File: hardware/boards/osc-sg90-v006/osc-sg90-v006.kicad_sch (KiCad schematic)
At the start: 31 parts, among them J1 Servo Input, J2 Motor, J3 Debug, J4 Potentiometer, U1 H7133-1_C277537, U4 DRV8837, U5 CH32V006F8U6, U6 74LVC2G241GS,115

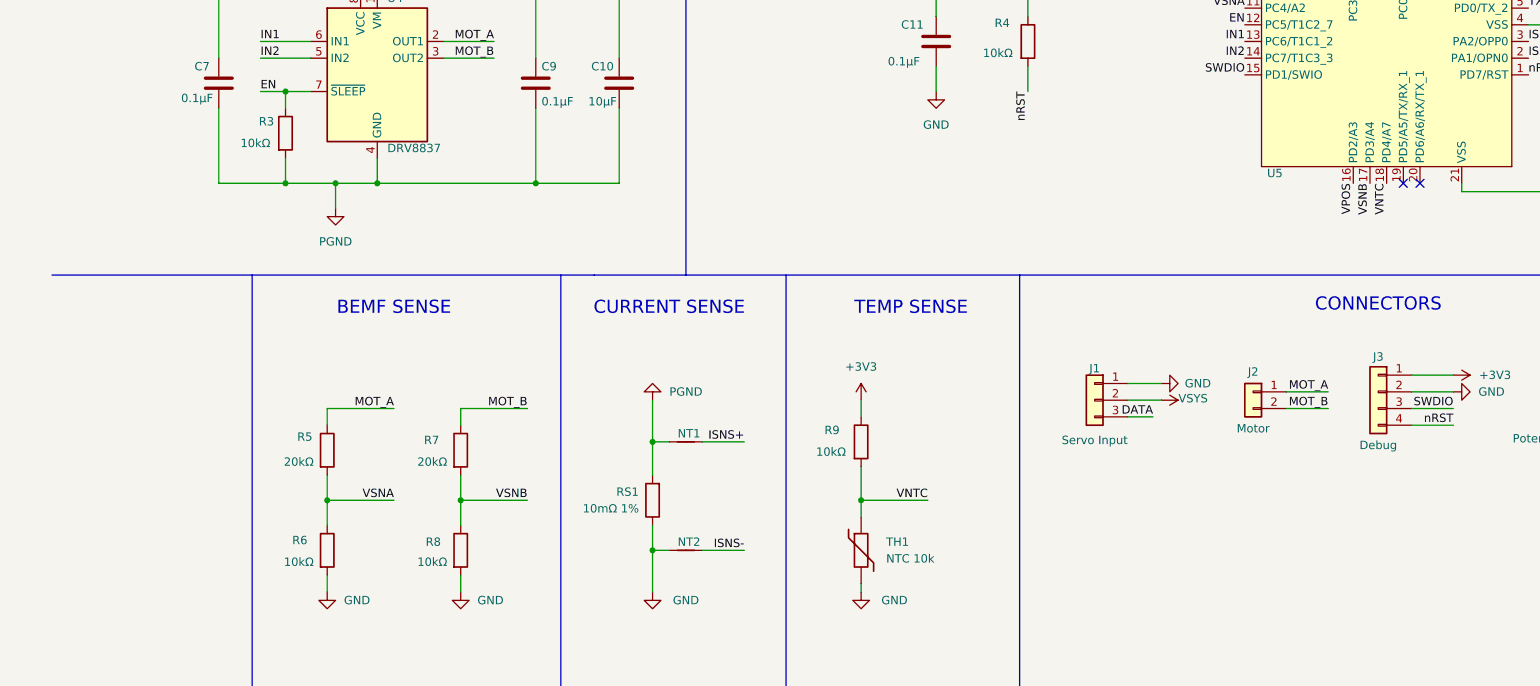
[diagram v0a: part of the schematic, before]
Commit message: update
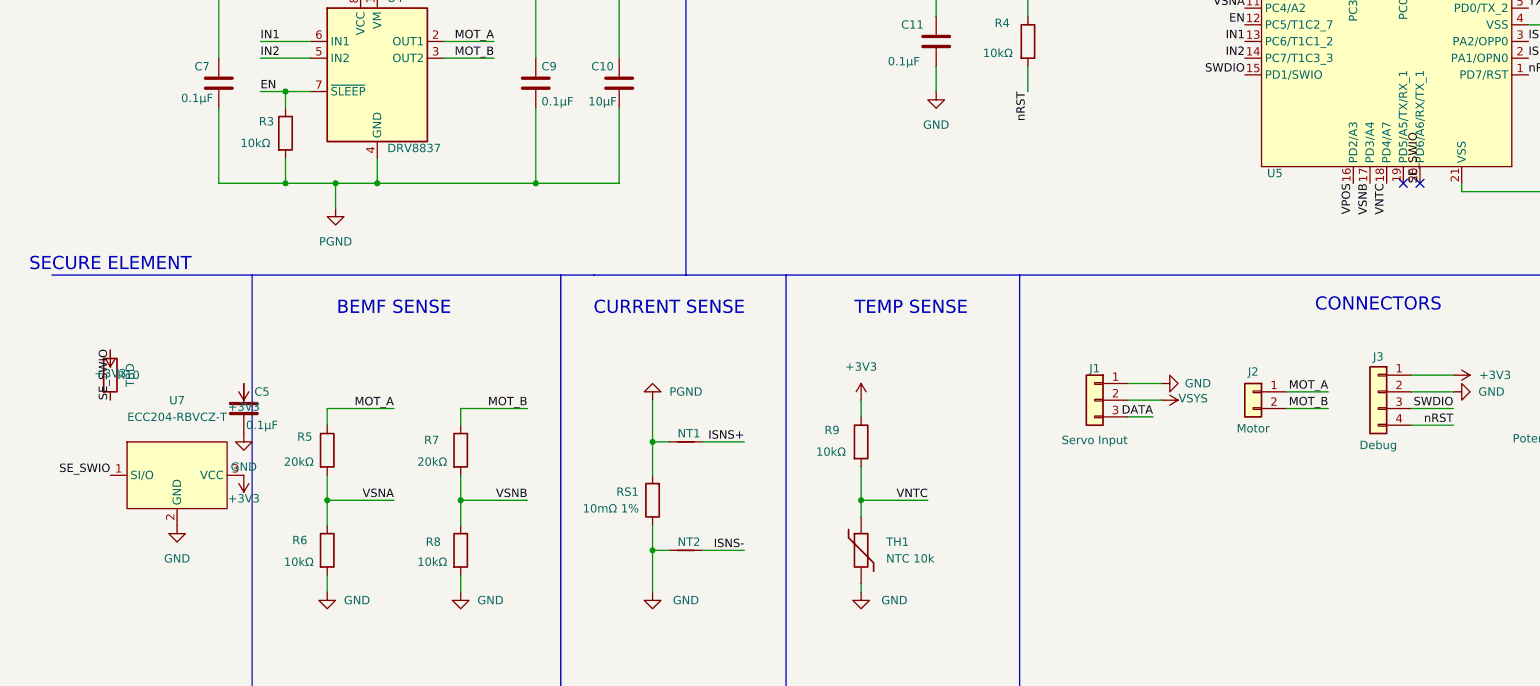
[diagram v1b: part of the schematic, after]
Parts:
- added C5: 0.1µF, Capacitor_SMD:C_0402_1005Metric, symbol Device:C
- added R10: TBD, Resistor_SMD:R_0402_1005Metric, symbol Device:R
- added U7: ECC204-RBVCZ-T, shared:ECC204_Contact-3_L6.5-W2.5-P2.00, symbol shared:ECC204-RBVCZ-T
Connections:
- net +3V3: now also C5.1, R10.1, U7.3 (VCC)
- net GND: now also C5.2, U7.2 (GND)
- net SE_SWIO: now reaches U5.20 (PD6/A6/RX/TX_1)
- net SE_SWIO: now also R10.2, U7.1 (SI/O)
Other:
- note added: "SECURE ELEMENT"

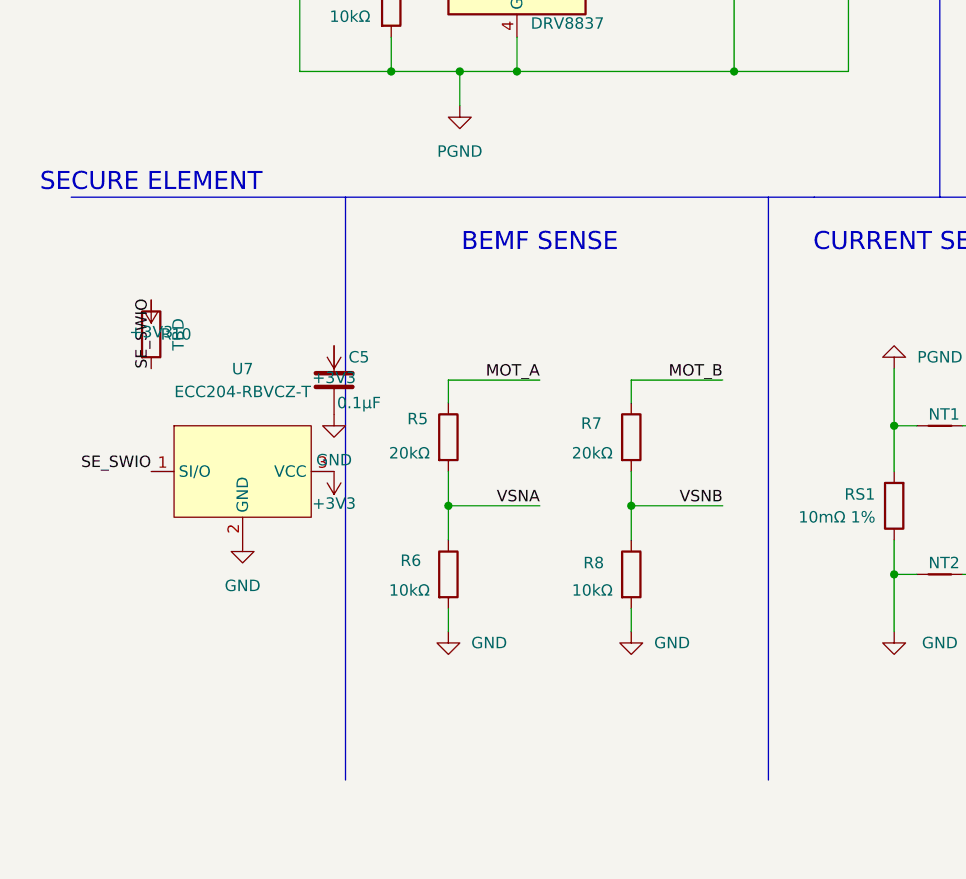
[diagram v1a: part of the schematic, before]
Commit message: cleaned up a lot of stuff
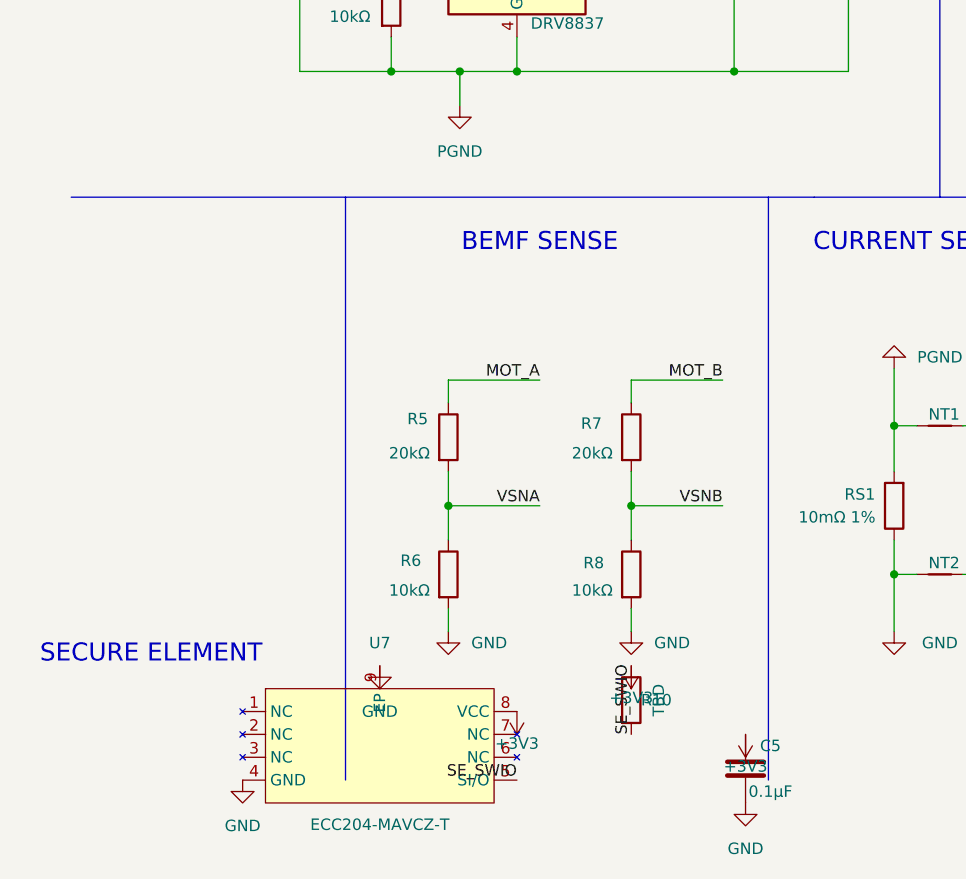
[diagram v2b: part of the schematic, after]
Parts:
- removed U7: ECC204-RBVCZ-T, shared:ECC204_Contact-3_L6.5-W2.5-P2.00, symbol shared:ECC204-RBVCZ-T
- added U7: ECC204-MAVCZ-T, shared:ECC204_UDFN-8-1EP_L2.0-W3.0-P0.50-EP0.61x1.3mm, symbol shared:ECC204-MAVCZ-T
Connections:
- net +3V3: now also U7.8 (VCC)
- net GND: now also U7.4 (GND), U7.9 (EP)
- net SE_SWIO: now also U7.5 (SI/O)
